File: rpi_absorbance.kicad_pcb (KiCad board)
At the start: 2 copper layers, 15 parts, among them P1 CONN_01X04, U1 LTC2461, U3 SD100-13-23-222, U4 OPA381

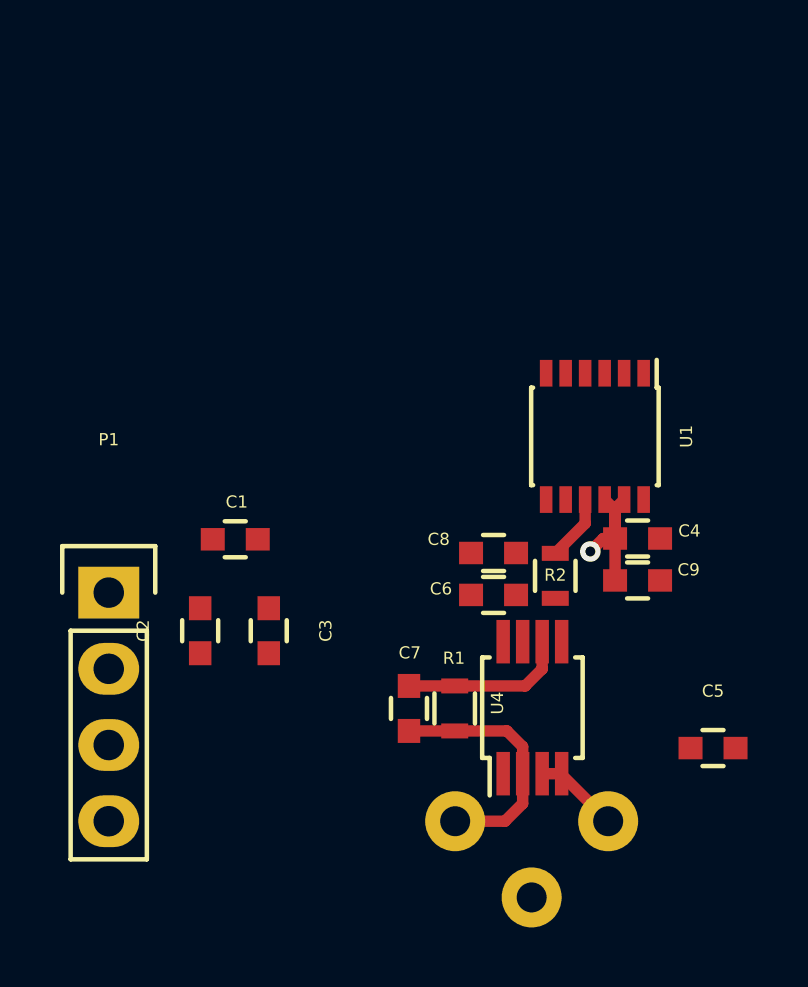
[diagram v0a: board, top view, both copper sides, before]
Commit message: Rearrange components
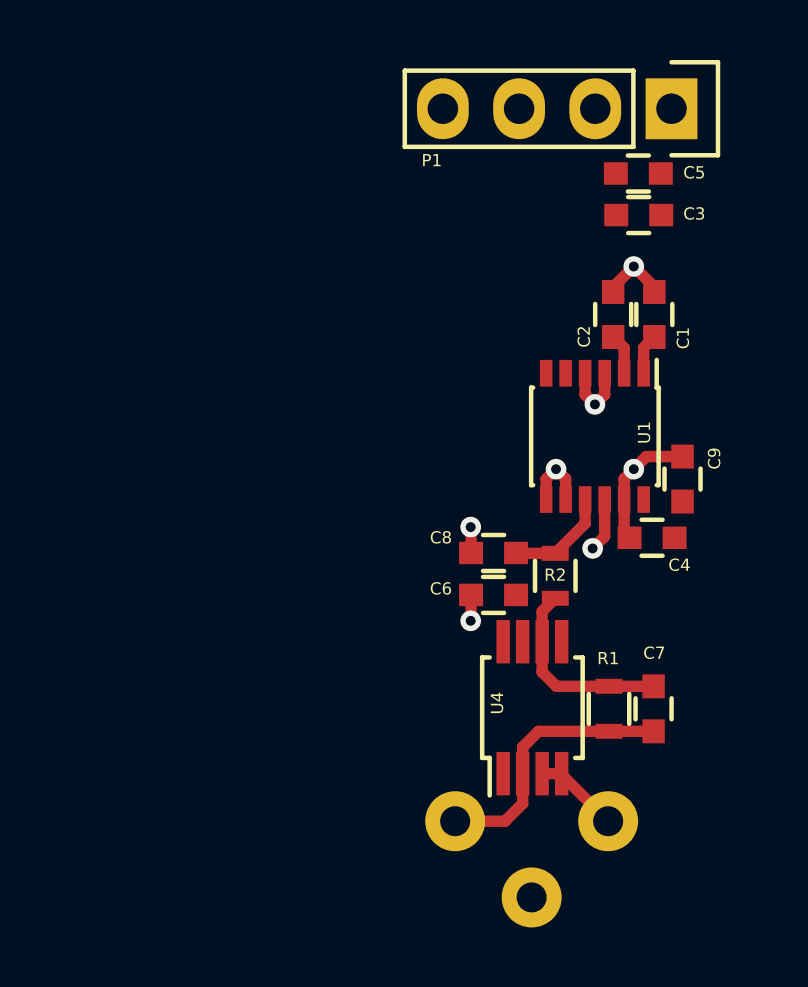
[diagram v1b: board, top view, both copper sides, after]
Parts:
- moved P1 24.7 mm to (138.6, 85.7), turned to 270 degrees
- moved C5 19.3 mm to (137.5, 87.9)
- moved C3 18.5 mm to (137.6, 89.3), turned to 0 degrees
- moved C2 17.3 mm to (136.7, 92.6)
- moved C1 15.9 mm to (138.1, 92.6), turned to 90 degrees
- moved C7 8.15 mm to (138.0, 105.7)
- moved R1 5.14 mm to (136.6, 105.7)
- moved C9 3.70 mm to (139.0, 98.1), turned to 270 degrees
- moved C4 0.48 mm to (138.0, 100.0)
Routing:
- net GND: track 8.14 -> 17.4 mm, vias 1 -> 7
- net Net-(C2-Pad1): track 0.00 -> 1.36 mm
- net Net-(C1-Pad1): track 0.00 -> 1.36 mm
- net Net-(C8-Pad1): track 2.21 -> 3.52 mm
- net Net-(C7-Pad1): track 5.58 -> 6.55 mm
- net Net-(C7-Pad2): track 8.40 -> 8.96 mm
